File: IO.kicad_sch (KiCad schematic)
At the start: 23 parts, among them Q4 S8050, Q5 IRF3708S, Q6 S8050, U13 LTV-817S, U14 LTV-817S

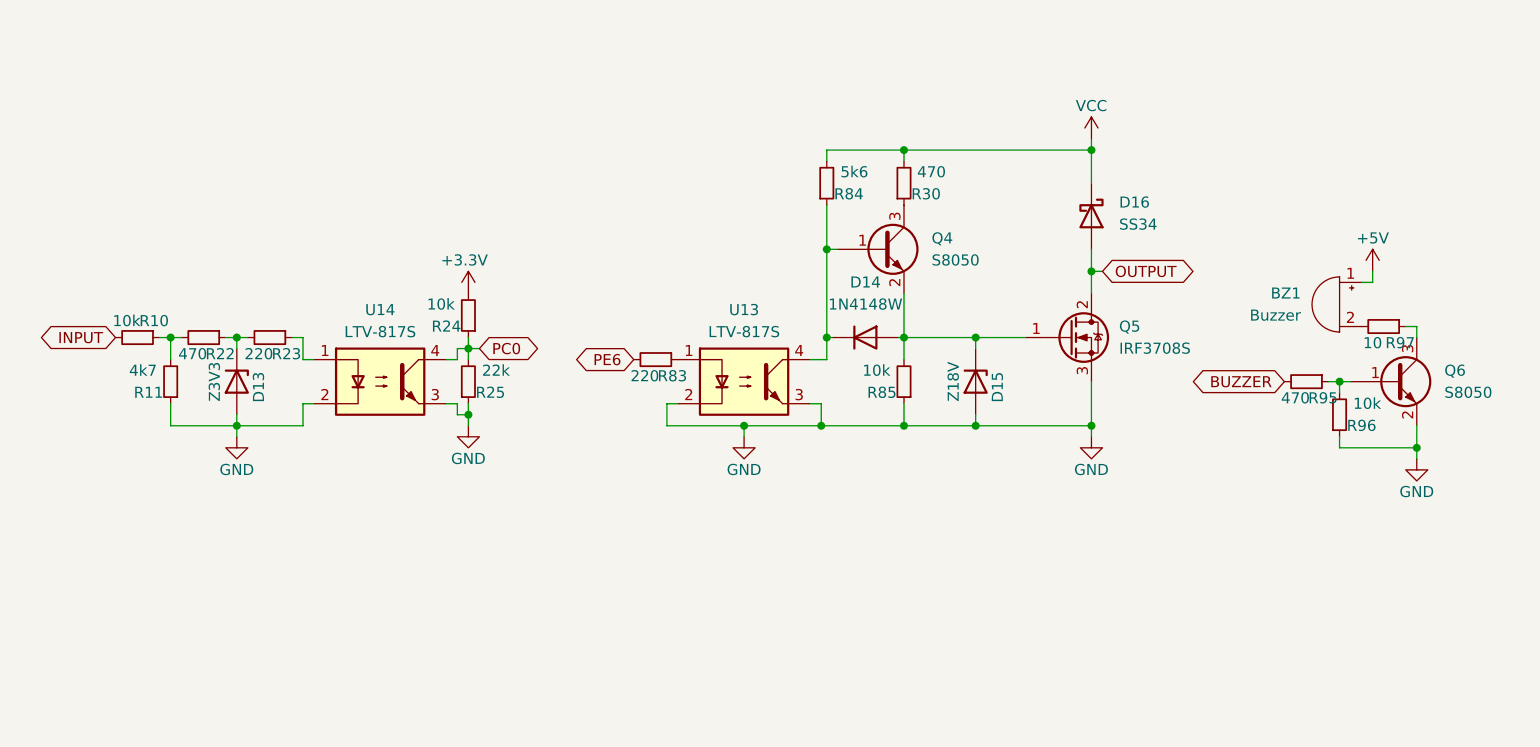
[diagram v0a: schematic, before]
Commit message: Add files via upload
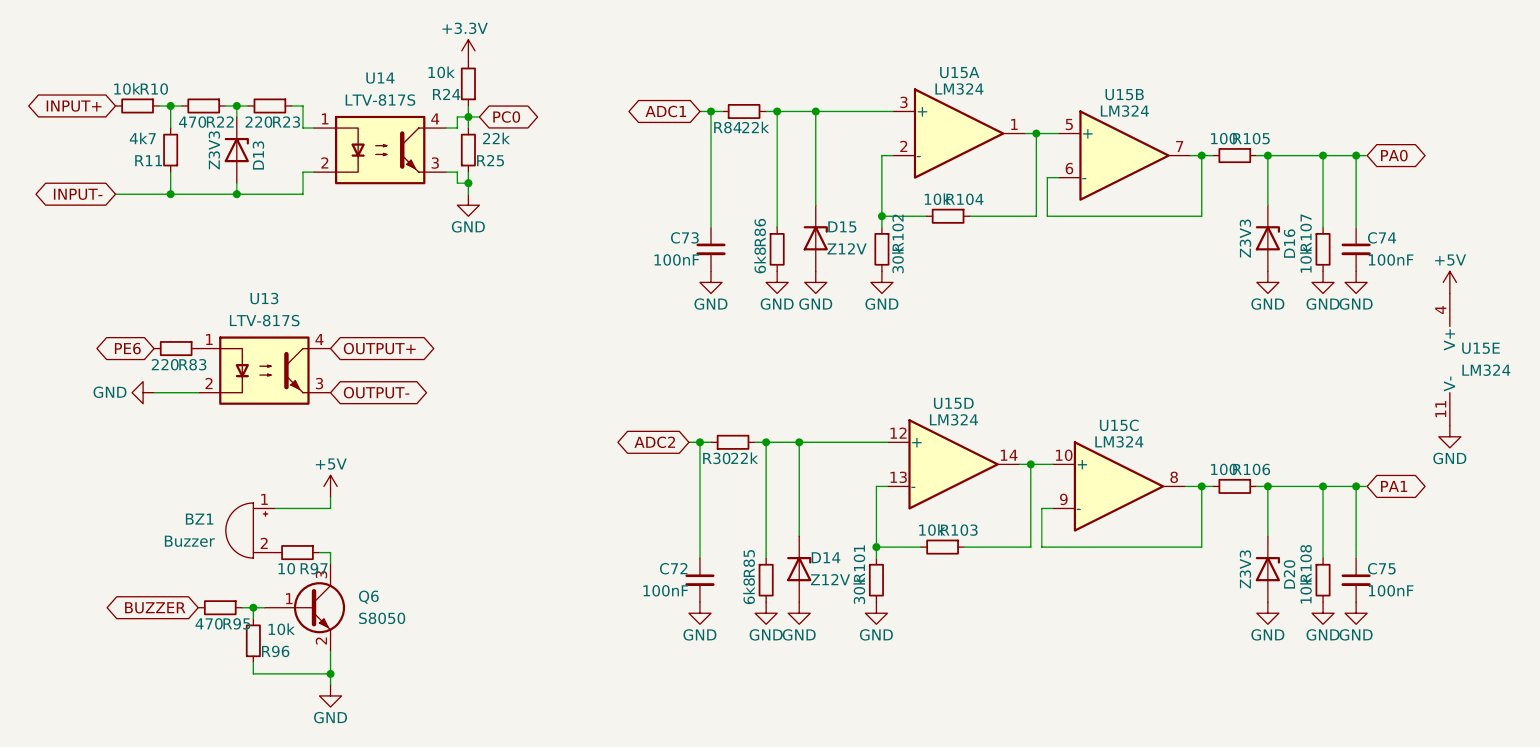
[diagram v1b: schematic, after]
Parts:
- removed D14: 1N4148W, Diode_SMD:D_SOD-123, symbol Diode:1N4148W
- removed D15: Z18V, Diode_SMD:D_SOD-123F, symbol Diode:BZV55C3V3
- removed D16: SS34, Diode_SMD:D_SMA, symbol Diode:CDBA340-HF
- removed Q4: S8050, Package_TO_SOT_SMD:SOT-23, symbol Transistor_BJT:BC847
- removed Q5: IRF3708S, Package_TO_SOT_SMD:TO-252-2, symbol Transistor_FET:QM6006D
- added C72, C73, C74, C75: 100nF, Capacitor_SMD:C_0603_1608Metric, symbol Device:C_Small
- added D14, D15: Z12V, Diode_SMD:D_SOD-123F, symbol Diode:BZV55B12
- added D16, D20: Z3V3, Diode_SMD:D_SOD-123F, symbol Diode:BZV55C3V3
- added R101, R102: 30k, Resistor_SMD:R_0603_1608Metric, symbol Device:R_Small
- added R103, R104, R107, R108: 10k, Resistor_SMD:R_0603_1608Metric, symbol Device:R_Small
- added R105, R106: 100, Resistor_SMD:R_0603_1608Metric, symbol Device:R_Small
- added R86: 6k8, Resistor_SMD:R_0603_1608Metric, symbol Device:R_Small
- added U15: LM324, Package_SO:SOIC-14_3.9x8.7mm_P1.27mm, symbol Amplifier_Operational:LM324
- R30: value 470 -> 22k
- R84: value 5k6 -> 22k
- R85: value 10k -> 6k8
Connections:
- net +5V: now also U15.4 (V+)
- net GND: now also R85.2, C72.2, C73.2, C74.2, C75.2, D14.2 (A), D15.2 (A), D16.2 (A), D20.2 (A), R101.2, R102.2, R107.2, R108.2, R86.2, U15.11 (V-); no longer D13.2 (A), R11.1, R85.1, U13.3, U14.2
- net ADC2: now reaches R30.1
- net ADC2: now also C72.1
- net ADC1: now reaches R84.1
- net ADC1: now also C73.1; no longer U13.4
- net INPUT renamed INPUT+
- net VCC: no longer names the net of R84.2
- net VCC: now also D15.1 (K), R86.1, U15.3 (+); no longer R30.2
- new net: R104.1, U15.1, U15.5 (+)
- new net: R102.1, R104.2, U15.2 (-)
- new net: D14.1 (K), R30.2, R85.1, U15.12 (+)
- new net: R103.1, U15.10 (+), U15.14
- new net: R101.1, R103.2, U15.13 (-)
- new net: R106.2, U15.8, U15.9 (-)
- new net: R105.2, U15.6 (-), U15.7
- new net INPUT-: D13.2 (A), R11.1, U14.2
- new net OUTPUT+: U13.4
- new net OUTPUT-: U13.3
- new net PA0: C74.1, D16.1 (K), R105.1, R107.1
- new net PA1: C75.1, D20.1 (K), R106.1, R108.1
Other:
- moved on the sheet: BZ1, D13, Q6, R10, R11, R22, R23, R24, R25, R83, R95, R96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
